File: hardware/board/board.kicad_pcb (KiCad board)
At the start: 4 copper layers, 300 x 120 mm, 239 parts, among them J201 LineOut, J202 Headphone, J203 LineIn, J301 MidiIn, J302 MidiOut, J501 USB_B_Micro, J502 USB_C_Receptacle_PowerOnly_6P, P501 USB_C_Plug_USB2.0, SW401 SW_Push, SW402 SW_Push, SW403 SW_Push, SW404 SW_Push, SW405 SW_Push, SW406 SW_Push, SW407 SW_Push, SW408 SW_Push, SW409 SW_Push, SW410 SW_Push, SW411 SW_Push, SW412 SW_Push, SW413 SW_Push, SW414 SW_Push, SW415 SW_Push, SW416 SW_Push, SW417 SW_Push, SW418 SW_Push, SW419 SW_Push, SW420 SW_Push, SW421 SW_Push, SW422 SW_Push, SW423 SW_Push, SW424 SW_Push, SW425 SW_Push, SW426 SW_Push, SW427 SW_Push, SW428 SW_Push, SW429 SW_Push, SW430 SW_Push, SW431 SW_Push, SW432 SW_Push, SW433 SW_Push, SW434 SW_Push, SW435 SW_Push, SW436 SW_Push, SW437 SW_Push, SW438 SW_Push, SW439 SW_Push, SW440 SW_Push, SW441 SW_Push, U101 Oled, U201 MAX98089ETN_T, U202 TPS7A20xxxDBV, U301 RP2350_80QFN, U302 THB001P, U303 TLP2310, U304 74AHC1G125DCKR, U501 AP22653W6, U502 FSUSB42MX, U503 TPS259531DSGR, Y201 12.288MHz, Y301 ABM8-272-T3

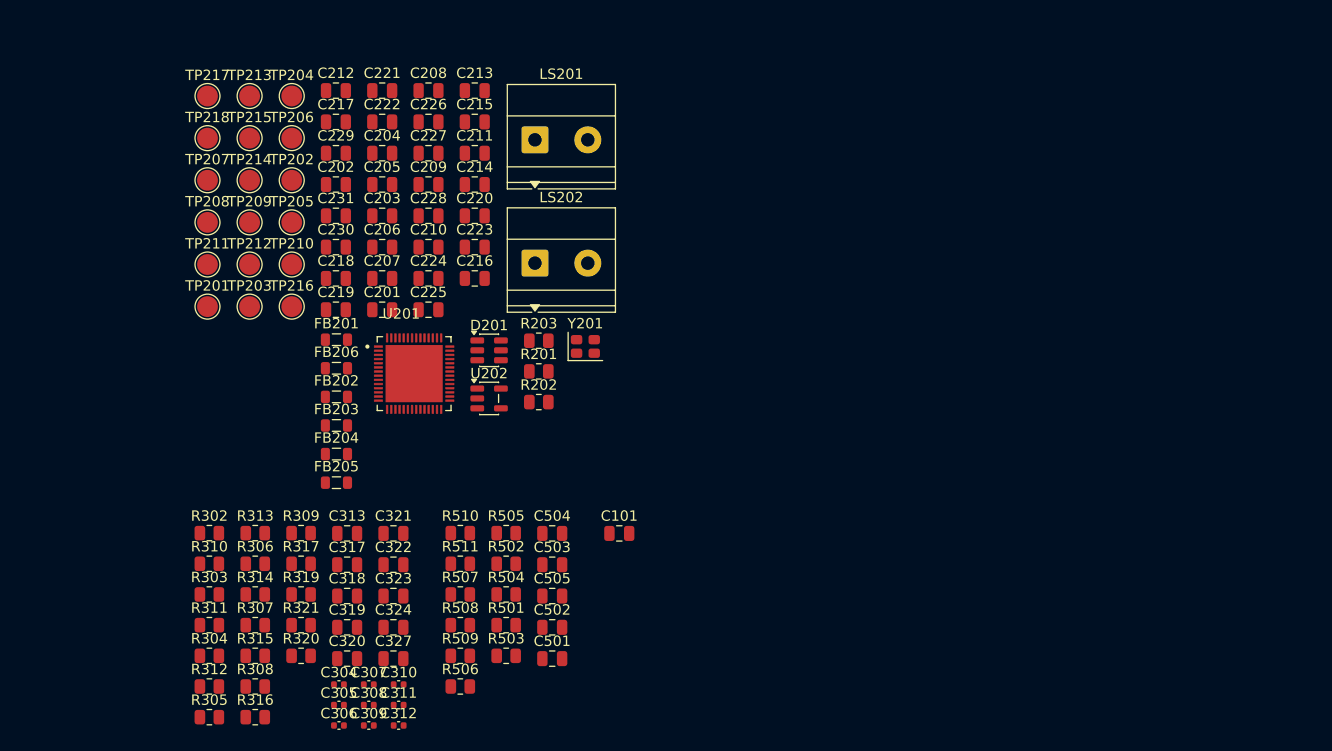
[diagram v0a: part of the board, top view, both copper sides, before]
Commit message: successfully got hat in?
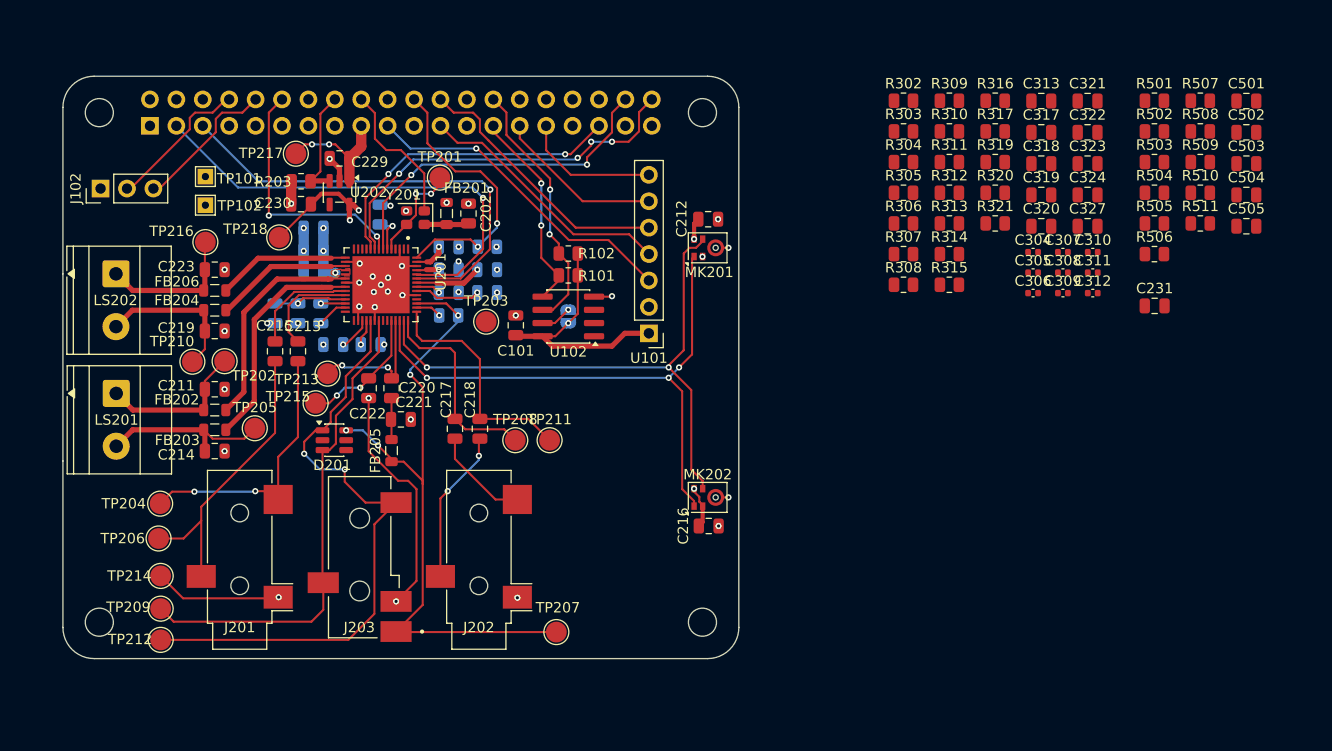
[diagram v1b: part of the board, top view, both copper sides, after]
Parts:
- added J101: CM4_DEBUG, Connector_PinSocket_2.54mm:PinSocket_2x20_P2.54mm_Vertical, B.Cu at (191.5, 221.9)
- added J102: DEBUG_PORT, Connector_PinHeader_2.54mm:PinHeader_1x03_P2.54mm_Vertical, F.Cu at (186.7, 227.9)
- added J201: LineOut, Connector_Audio:Jack_3.5mm_CUI_SJ-3523-SMT_Horizontal, F.Cu at (200.1, 263.6)
- added J202: LineIn, Connector_Audio:Jack_3.5mm_CUI_SJ-3523-SMT_Horizontal, F.Cu at (223.1, 263.6)
- added J203: Headphone, footprints:CUI_SJ-43514-SMT-TR, F.Cu at (215.2, 270.5)
- added JP101: ID_WP, Jumper:SolderJumper-2_P1.3mm_Open_RoundedPad1.0x1.5mm, B.Cu at (231.7, 240.2)
- added MH1: MountingHole_2.7mm_M2.5, MountingHole:MountingHole_2.7mm_M2.5, F.Cu at (186.6, 220.6)
- added MH2: MountingHole_2.7mm_M2.5, MountingHole:MountingHole_2.7mm_M2.5, F.Cu at (244.6, 220.6)
- added MH3: MountingHole_2.7mm_M2.5, MountingHole:MountingHole_2.7mm_M2.5, F.Cu at (186.6, 269.6)
- added MH4: MountingHole_2.7mm_M2.5, MountingHole:MountingHole_2.7mm_M2.5, F.Cu at (244.6, 269.6)
- added MK201: MicL, Sensor_Audio:Knowles_LGA-5_3.5x2.65mm, F.Cu at (245.1, 233.6)
- added MK202: MicR, Sensor_Audio:Knowles_LGA-5_3.5x2.65mm, F.Cu at (245.1, 257.6)
- added R101: 3.9k, Resistor_SMD:R_0805_2012Metric, F.Cu at (231.7, 236.3)
- added R102: 3.9k, Resistor_SMD:R_0805_2012Metric, F.Cu at (231.7, 234.2)
- added TP101: 5V, TestPoint:TestPoint_THTPad_1.5x1.5mm_Drill0.7mm, F.Cu at (196.8, 226.8)
- added TP102: GND, TestPoint:TestPoint_THTPad_1.5x1.5mm_Drill0.7mm, F.Cu at (196.8, 229.5)
- added U101: Oled, Connector_PinHeader_2.54mm:PinHeader_1x07_P2.54mm_Vertical, F.Cu at (239.5, 241.8)
- added U102: CAT24C256, Package_SO:SOIC-8_3.9x4.9mm_P1.27mm, F.Cu at (231.7, 240.2)
- C201, C203, C204, C205, C206, C207, C208, C209, C210, C224, C225, C226, C227, C228, R201, R202: moved to B.Cu
- moved R316 92.6 mm to (272.8, 219.5)
- moved C501 85.6 mm to (296.9, 219.5)
- moved R312 85.5 mm to (268.4, 228.3)
- moved R509 85.5 mm to (292.5, 225.4)
- moved R507 85.5 mm to (292.5, 219.5)
- moved R508 85.5 mm to (292.5, 222.4)
- moved R311 83.9 mm to (268.4, 225.4)
- moved R305 83.7 mm to (264.0, 228.3)
- moved R310 82.4 mm to (268.4, 222.4)
- moved C502 82.0 mm to (296.9, 222.5)
- moved R304 81.9 mm to (264.0, 225.4)
- moved R320 80.2 mm to (272.8, 228.3)
- moved R303 80.2 mm to (264.0, 222.4)
- moved R501 80.2 mm to (288.1, 219.5)
- moved C231 79.2 mm to (288.1, 239.2)
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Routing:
- net GND: track 3.53 -> 93.5 mm, vias 5 -> 46
- net /codec/JackS: track 0.00 -> 63.6 mm
- net Net-(D201-TVS1): track 0.00 -> 60.5 mm, vias 0 -> 2
- net /audio/DIGMICDATA: track 0.00 -> 55.9 mm, vias 0 -> 3
- net /audio/DIGMICCLK: track 0.00 -> 55.8 mm, vias 0 -> 2
- net Net-(D201-TVS2): track 0.00 -> 47.1 mm
- net /GPIO2/SDA1: track 0.00 -> 44.7 mm
- net /I2C1_SCL: track 0.00 -> 44.1 mm, vias 0 -> 1
- net +3V3: track 0.00 -> 42.3 mm, vias 0 -> 7
- net /PCM_DOUT: track 0.00 -> 37.2 mm, vias 0 -> 4
- net +1V8: track 0.00 -> 34.9 mm, vias 0 -> 7
- net /PCM_FS: track 0.00 -> 33.4 mm, vias 0 -> 2
- net /GPIO10/SPI0.MOSI: track 0.00 -> 31.3 mm, vias 0 -> 1
- net /PCM_DIN: track 0.00 -> 30.5 mm, vias 0 -> 2
- net Net-(C215-Pad2): track 0.00 -> 28.4 mm
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- added copper zone on In2.Cu, net +1V8
- added copper zone on In2.Cu, net +3V3
- added copper zone on F.Cu, net +5V
- added copper zone on In2.Cu, net +5V
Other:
- board size 300 x 120 mm -> 300 x 189.6 mm
- board text added: "PoE"
- board text added: "RJ45"
